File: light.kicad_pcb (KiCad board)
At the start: 2 copper layers, 29.2 x 18.2 mm, 7 parts, among them P1 CONN_01X02, U1 TSL252, U2 LF50CV-DG

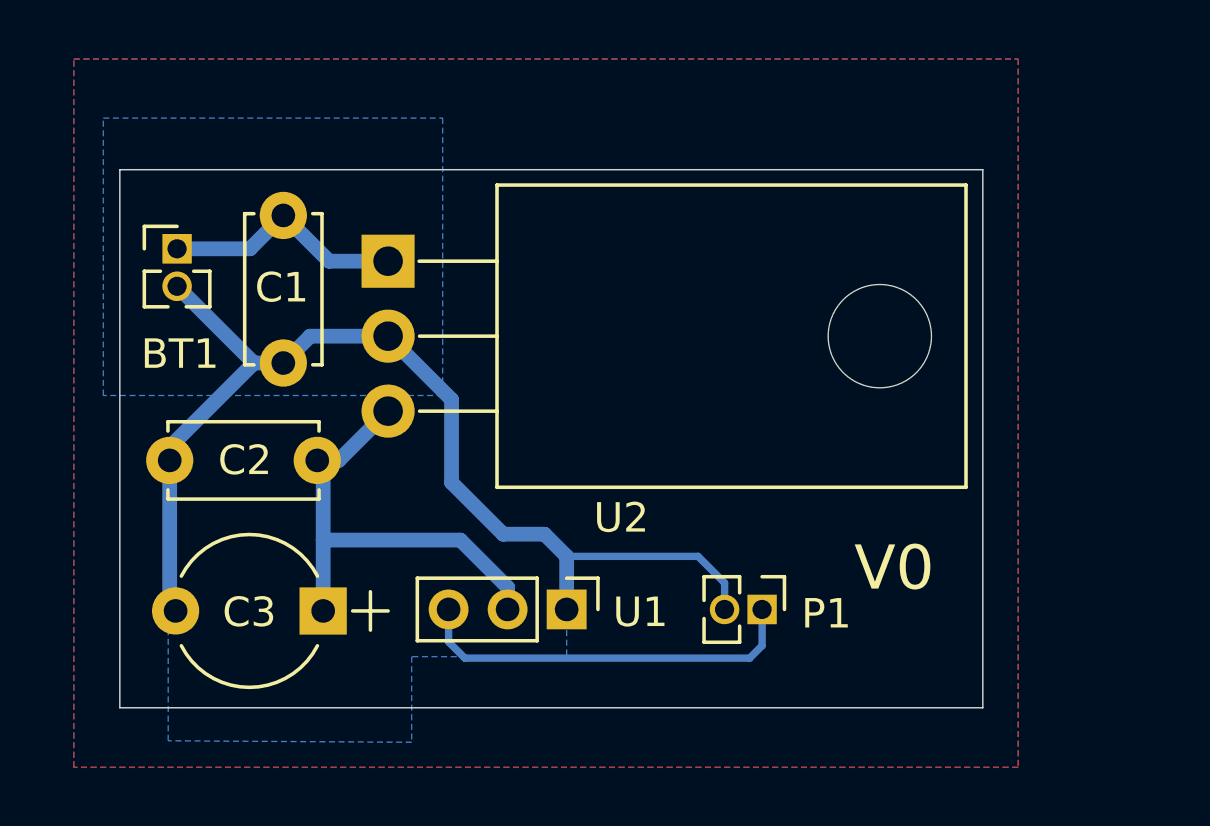
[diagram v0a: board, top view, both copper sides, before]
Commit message: Board V1 should be done. Ready for fab?
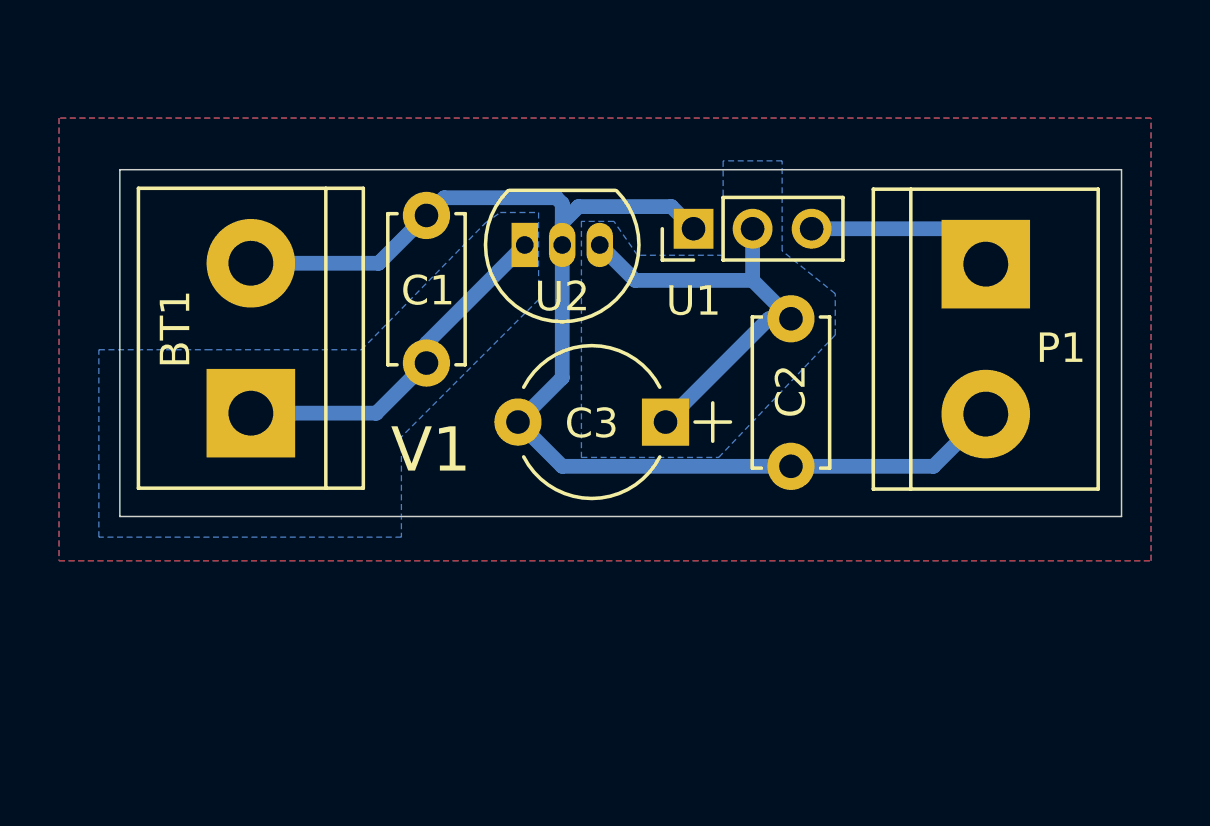
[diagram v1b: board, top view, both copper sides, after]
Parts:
- BT1, P1: footprint Pin_Headers:Pin_Header_Straight_1x02_Pitch1.27mm -> Connectors_Terminal_Blocks:TerminalBlock_bornier-2_P5.08mm
- U2: value LF50CV-DG -> LM340LAZ-5.0/NOPB; footprint TO_SOT_Packages_THT:TO-220-3_Horizontal -> Customs:TO-92_Inline_Narrow_Flip
- moved C2 16.8 mm to (158.3, 91.8), turned to 270 degrees
- moved P1 13.9 mm to (164.9, 90.0)
- moved U1 13.6 mm to (155.0, 88.8), turned to 90 degrees
- moved C3 13.2 mm to (154.1, 95.3)
- moved C1 6.97 mm to (145.9, 93.3), turned to 90 degrees
- moved BT1 6.11 mm to (140.0, 95.0), turned to 90 degrees
- moved U2 5.93 mm to (150.6, 89.3), turned to 180 degrees
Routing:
- net Net-(P1-Pad1): track 13.4 -> 6.40 mm
- net GND: track 37.5 -> 42.5 mm
- net +BATT: track 8.26 -> 12.0 mm
- net +5V: track 15.9 -> 15.0 mm
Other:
- board size 29.2 x 18.2 mm -> 33.9 x 11.8 mm
- board text added: "V1"
- board text removed: "V0"
